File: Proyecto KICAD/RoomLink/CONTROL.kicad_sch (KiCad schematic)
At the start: 15 parts, among them U10 ESP32-WROOM-32

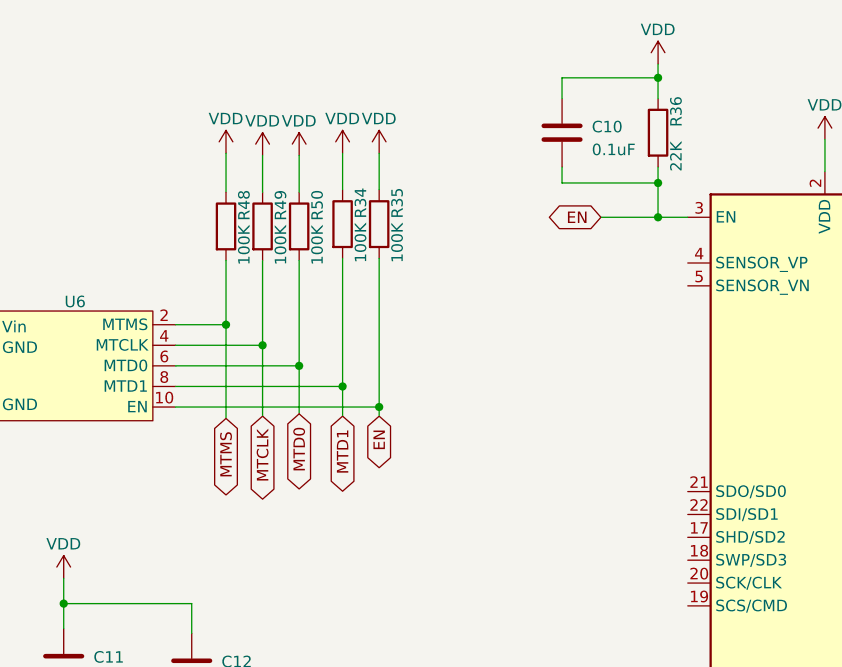
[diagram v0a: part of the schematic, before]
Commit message: ll
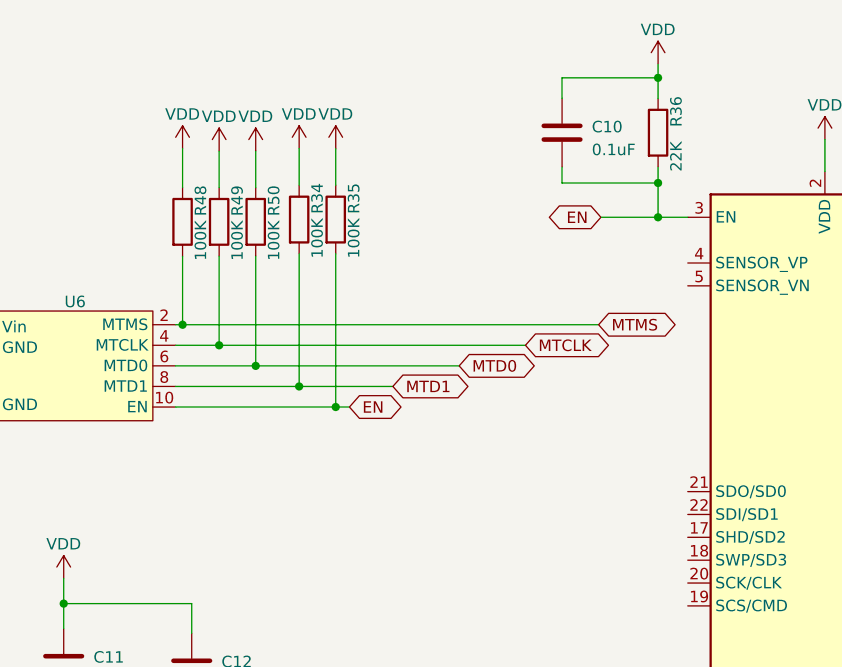
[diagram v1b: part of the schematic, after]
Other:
- moved on the sheet: R34, R35, R48, R49, R50
